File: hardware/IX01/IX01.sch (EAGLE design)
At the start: 14 parts, among them IC1 P82B715, IC2 P82B715

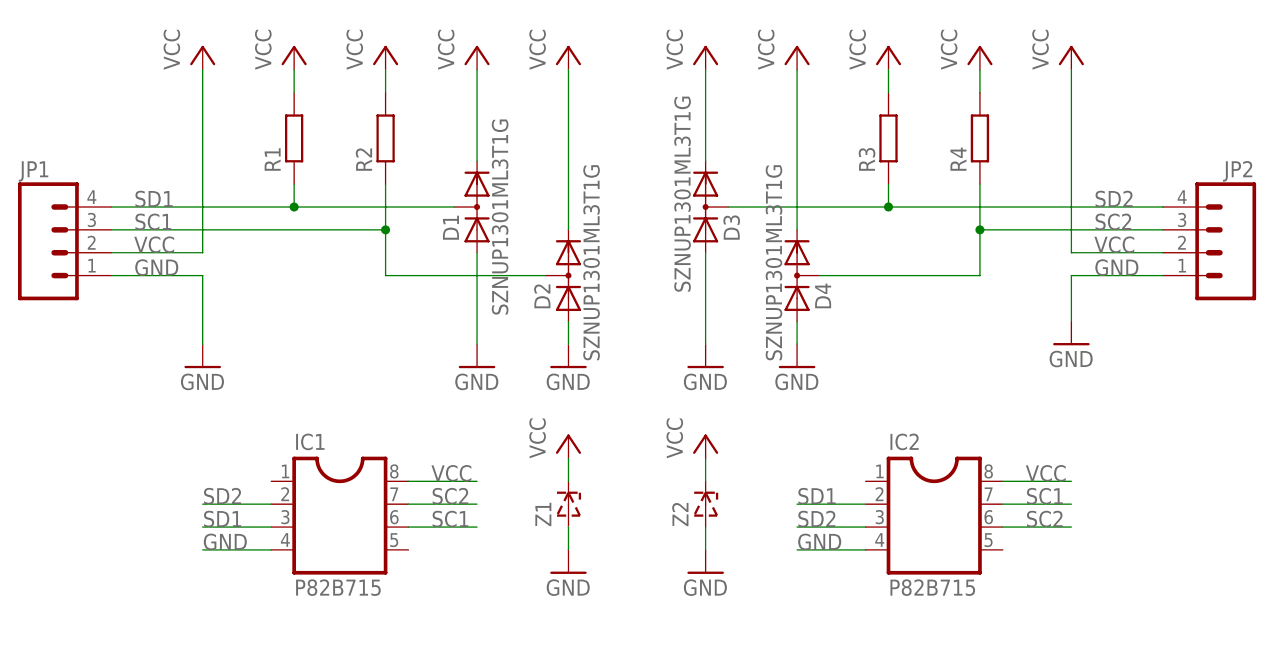
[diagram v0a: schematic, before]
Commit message: IX01 for Seeedstudio
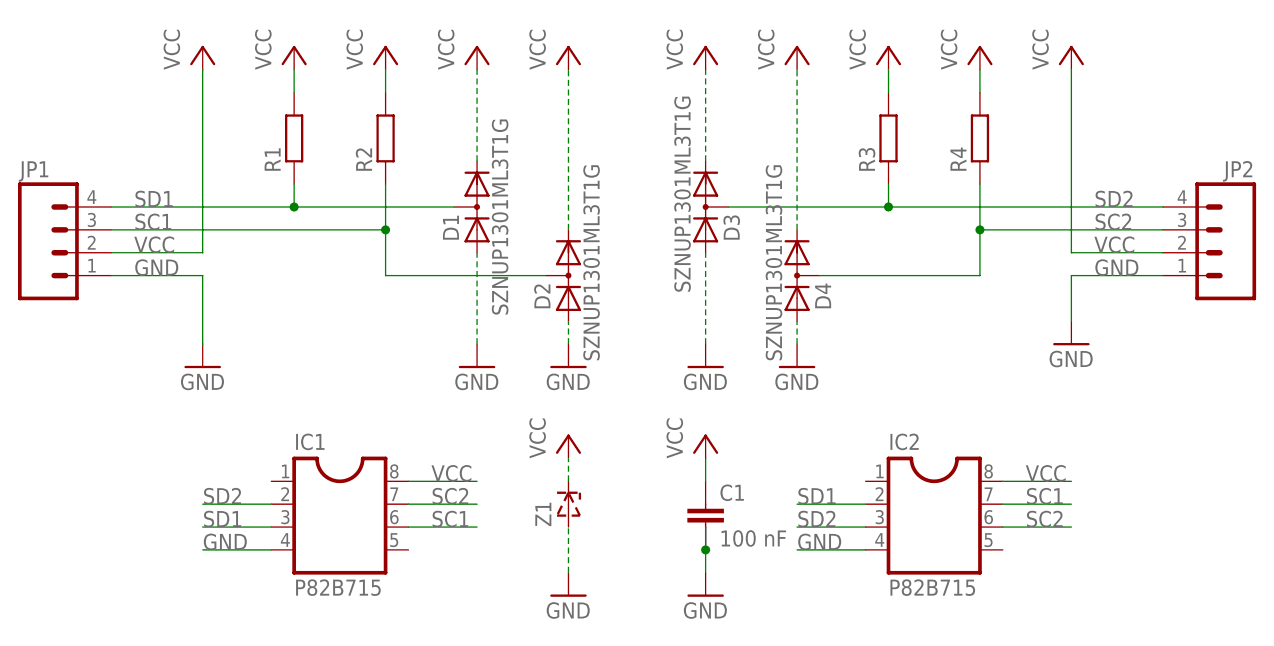
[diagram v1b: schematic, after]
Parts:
- removed Z2: (no value), dp_devices:ZENERSOD-323F
- added C1: 100 nF, rcl:C-EUC0805
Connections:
- net GND: now also C1.2; no longer Z2.A
- net VCC: now also C1.1; no longer Z2.C
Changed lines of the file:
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@@
 <part name="P+11" library="supply1" deviceset="VCC" device=""/>
 <part name="GND7" library="supply1" deviceset="GND" device=""/>
-<part name="Z2" library="dp_devices" deviceset="ZENER" device="SOD-323F"/>
 <part name="P+12" library="supply1" deviceset="VCC" device=""/>
 <part name="GND8" library="supply1" deviceset="GND" device=""/>
+<part name="C1" library="rcl" deviceset="C-EU" device="C0805" value="100 nF"/>
 </parts>
 <sheets>
@@
 <instance part="Z1" gate="G$1" x="-2.54" y="60.96" rot="R90"/>
 <instance part="P+11" gate="VCC" x="-2.54" y="68.58"/>
-<instance part="GND7" gate="1" x="-2.54" y="53.34"/>
-<instance part="Z2" gate="G$1" x="12.7" y="60.96" rot="R90"/>
+<instance part="GND7" gate="1" x="-2.54" y="50.8"/>
 <instance part="P+12" gate="VCC" x="12.7" y="68.58"/>
-<instance part="GND8" gate="1" x="12.7" y="53.34"/>
+<instance part="GND8" gate="1" x="12.7" y="50.8"/>
+<instance part="C1" gate="G$1" x="12.7" y="60.96"/>
 </instances>
 <busses>
@@
 <pinref part="GND3" gate="1" pin="GND"/>
 <pinref part="D1" gate="G$1" pin="A"/>
-<wire x1="-12.7" y1="78.74" x2="-12.7" y2="88.9" width="0.1524" layer="91"/>
+<wire x1="-12.7" y1="78.74" x2="-12.7" y2="88.9" width="0.1524" layer="91" style="shortdash"/>
 </segment>
 <segment>
 <pinref part="GND4" gate="1" pin="GND"/>
 <pinref part="D2" gate="G$1" pin="A"/>
-<wire x1="-2.54" y1="78.74" x2="-2.54" y2="81.28" width="0.1524" layer="91"/>
+<wire x1="-2.54" y1="78.74" x2="-2.54" y2="81.28" width="0.1524" layer="91" style="shortdash"/>
 </segment>
 <segment>
 <pinref part="GND5" gate="1" pin="GND"/>
 <pinref part="D3" gate="G$1" pin="A"/>
-<wire x1="12.7" y1="78.74" x2="12.7" y2="88.9" width="0.1524" layer="91"/>
+<wire x1="12.7" y1="78.74" x2="12.7" y2="88.9" width="0.1524" layer="91" style="shortdash"/>
 </segment>
 <segment>
 <pinref part="GND6" gate="1" pin="GND"/>
 <pinref part="D4" gate="G$1" pin="A"/>
-<wire x1="22.86" y1="78.74" x2="22.86" y2="81.28" width="0.1524" layer="91"/>
+<wire x1="22.86" y1="78.74" x2="22.86" y2="81.28" width="0.1524" layer="91" style="shortdash"/>
 </segment>
 <segment>
 <pinref part="GND7" gate="1" pin="GND"/>
 <pinref part="Z1" gate="G$1" pin="A"/>
-<wire x1="-2.54" y1="55.88" x2="-2.54" y2="58.42" width="0.1524" layer="91"/>
+<wire x1="-2.54" y1="53.34" x2="-2.54" y2="58.42" width="0.1524" layer="91" style="shortdash"/>
 </segment>
 <segment>
 <pinref part="GND8" gate="1" pin="GND"/>
-<pinref part="Z2" gate="G$1" pin="A"/>
+<wire x1="12.7" y1="53.34" x2="12.7" y2="55.88" width="0.1524" layer="91"/>
+<pinref part="C1" gate="G$1" pin="2"/>
 <wire x1="12.7" y1="55.88" x2="12.7" y2="58.42" width="0.1524" layer="91"/>
+<junction x="12.7" y="55.88"/>
 </segment>
 </net>
@@
 <pinref part="D1" gate="G$1" pin="C"/>
 <pinref part="P+7" gate="VCC" pin="VCC"/>
-<wire x1="-12.7" y1="99.06" x2="-12.7" y2="109.22" width="0.1524" layer="91"/>
+<wire x1="-12.7" y1="99.06" x2="-12.7" y2="109.22" width="0.1524" layer="91" style="shortdash"/>
 </segment>
 <segment>
 <pinref part="D2" gate="G$1" pin="C"/>
 <pinref part="P+8" gate="VCC" pin="VCC"/>
-<wire x1="-2.54" y1="91.44" x2="-2.54" y2="109.22" width="0.1524" layer="91"/>
+<wire x1="-2.54" y1="91.44" x2="-2.54" y2="109.22" width="0.1524" layer="91" style="shortdash"/>
 </segment>
 <segment>
 <pinref part="D3" gate="G$1" pin="C"/>
 <pinref part="P+9" gate="VCC" pin="VCC"/>
-<wire x1="12.7" y1="99.06" x2="12.7" y2="109.22" width="0.1524" layer="91"/>
+<wire x1="12.7" y1="99.06" x2="12.7" y2="109.22" width="0.1524" layer="91" style="shortdash"/>
 </segment>
 <segment>
 <pinref part="D4" gate="G$1" pin="C"/>
 <pinref part="P+10" gate="VCC" pin="VCC"/>
-<wire x1="22.86" y1="91.44" x2="22.86" y2="109.22" width="0.1524" layer="91"/>
+<wire x1="22.86" y1="91.44" x2="22.86" y2="109.22" width="0.1524" layer="91" style="shortdash"/>
 </segment>
 <segment>
 <pinref part="Z1" gate="G$1" pin="C"/>
 <pinref part="P+11" gate="VCC" pin="VCC"/>
-<wire x1="-2.54" y1="63.5" x2="-2.54" y2="66.04" width="0.1524" layer="91"/>
+<wire x1="-2.54" y1="63.5" x2="-2.54" y2="66.04" width="0.1524" layer="91" style="shortdash"/>
 </segment>
 <segment>
-<pinref part="Z2" gate="G$1" pin="C"/>
 <pinref part="P+12" gate="VCC" pin="VCC"/>
 <wire x1="12.7" y1="63.5" x2="12.7" y2="66.04" width="0.1524" layer="91"/>
+<pinref part="C1" gate="G$1" pin="1"/>
 </segment>
 </net>
